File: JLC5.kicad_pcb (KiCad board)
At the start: 2 copper layers, 101.9 x 102 mm, 123 parts, among them J1 Conn_01x05_Pin, J1 Conn_01x06_Pin, J1 Conn_01x12_Pin, J1 IPS_display, J1 SPEAKER, J1 USB_A, J2 Conn_01x02_Socket, J2 INPUT, SW1 SW_Push, SW1 SW_SPDT, SW2 SW_DIP_x02, U1 74HC595, U1 ATtiny85, U1 TC78H621FNG, U1 TPA3128D2, U2 CAT24C256, U2 EEPROM SOCKET, U2 TC78H621FNG, U3 TC78H621FNG, U4 TC78H621FNG, U5 74HC595

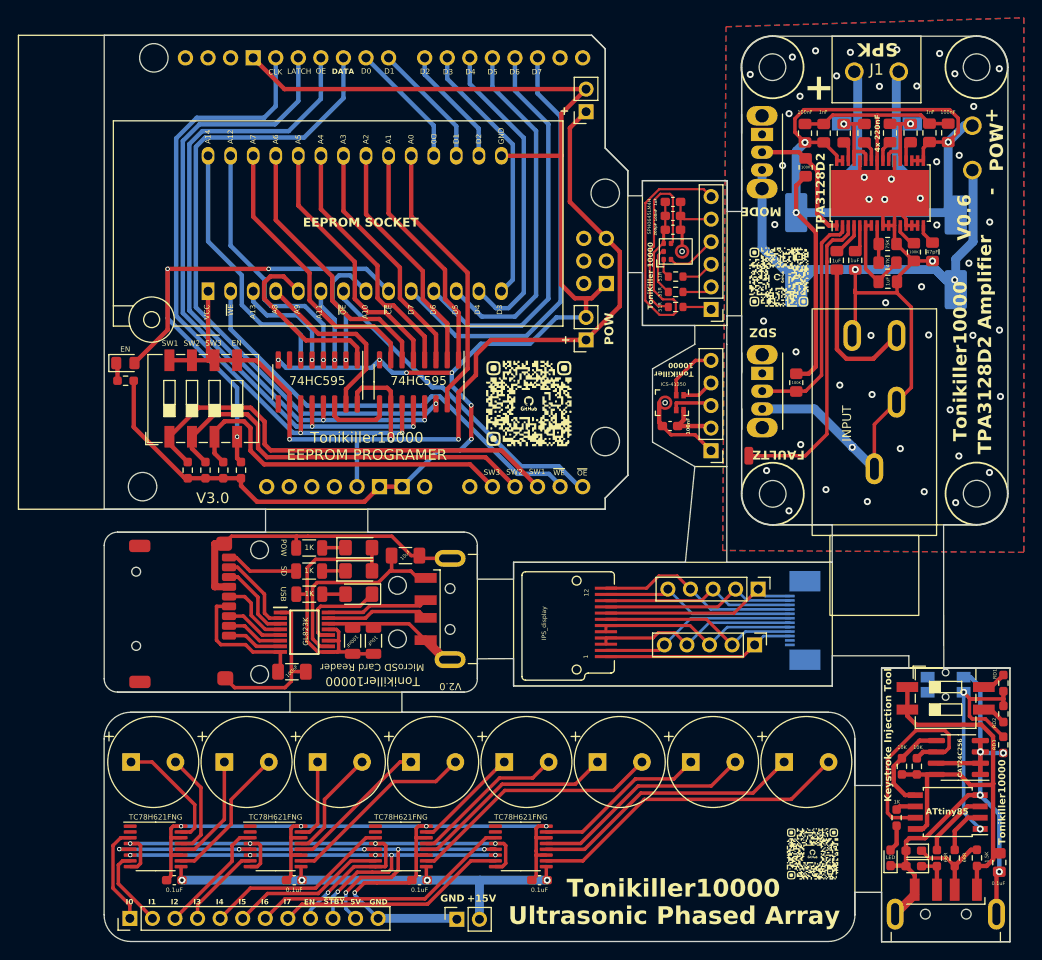
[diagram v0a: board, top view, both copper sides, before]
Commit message: f
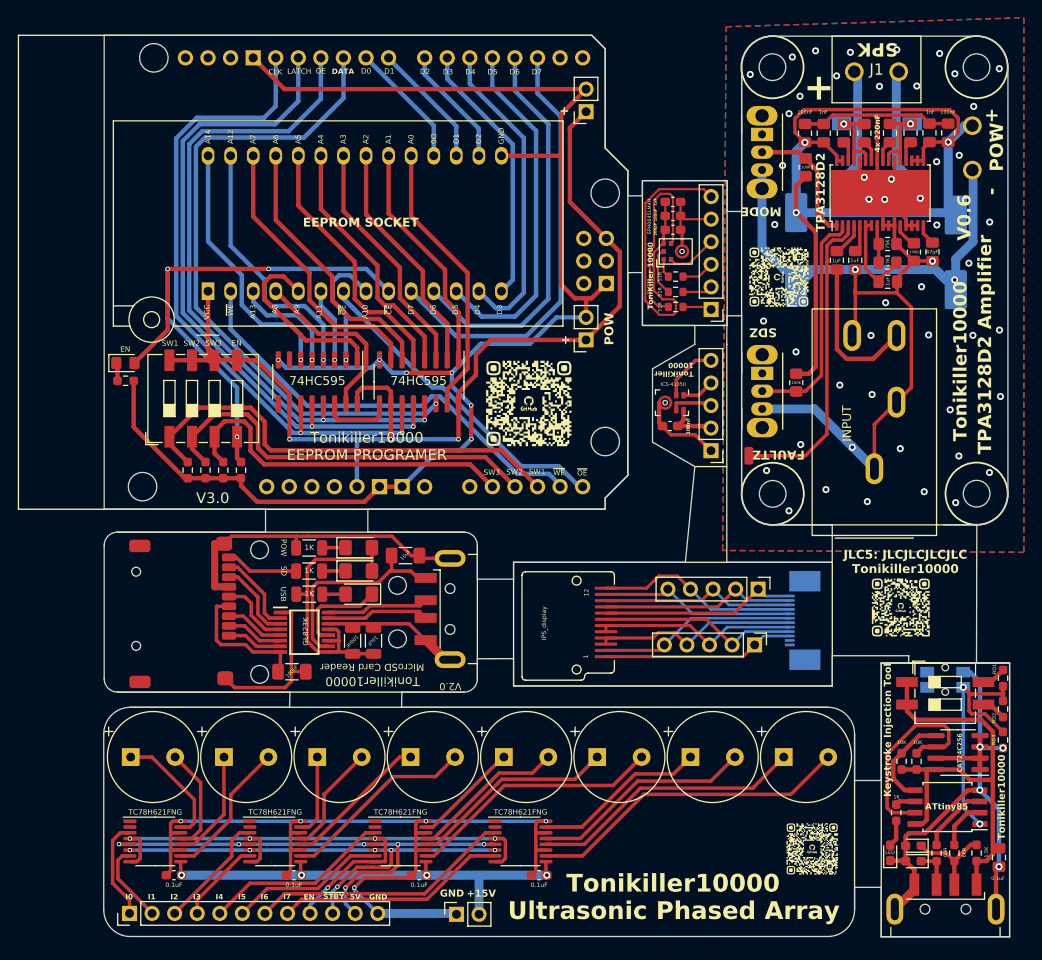
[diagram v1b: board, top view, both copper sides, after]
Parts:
- added G***: LOGO, LOGO, F.Cu at (239.2, 103.8)
- moved D3 0.56 mm to (237.9, 131.4)
- moved J1 0.56 mm to (244.2, 144.6)
- moved R1 0.56 mm to (245.2, 131.4)
- moved R2 0.56 mm to (243.2, 131.4)
- moved R3 0.56 mm to (247.7, 131.4)
- moved R4 0.56 mm to (239.2, 121.1)
- moved R9 0.56 mm to (250.6, 118.7)
- moved U1 0.56 mm to (155.2, 130.1)
- moved U1 0.56 mm to (244.4, 126.2)
- moved U2 0.56 mm to (168.7, 130.1)
- moved C1 0.56 mm to (157.3, 133.9)
- moved C1 0.56 mm to (250.2, 131.9)
- moved C2 0.56 mm to (170.8, 133.9)
- moved C3 0.56 mm to (184.9, 133.9)
- moved C4 0.56 mm to (198.4, 133.9)
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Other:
- board size 101.9 x 102 mm -> 101.9 x 101.5 mm
- board text added: "JLC5: JLCJLCJLCJLC Tonikiller10000"
